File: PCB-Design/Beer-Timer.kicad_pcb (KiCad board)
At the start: 2 copper layers, 47.5 x 19 mm, 19 parts, among them J1 Power, J2 Programmer Pins, J3 TM1637 4 Digit Display, J4 SOIC-ATtiny85-20U, J5 SOIC-2, J6 Switches, SW1 SW_SPDT, U1 MCP1700x-330xxTT, U2 ATtiny85-20S

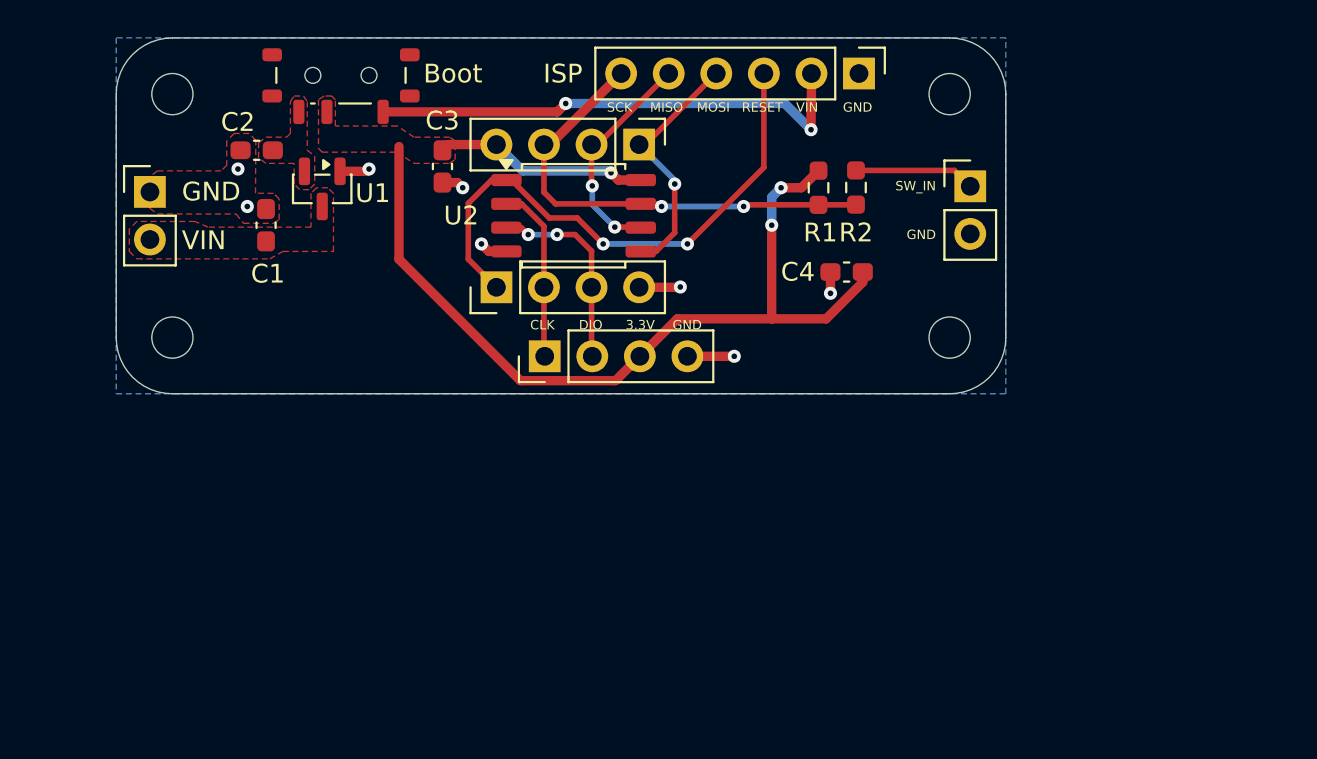
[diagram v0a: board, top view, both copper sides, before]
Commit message: Final PCB changes
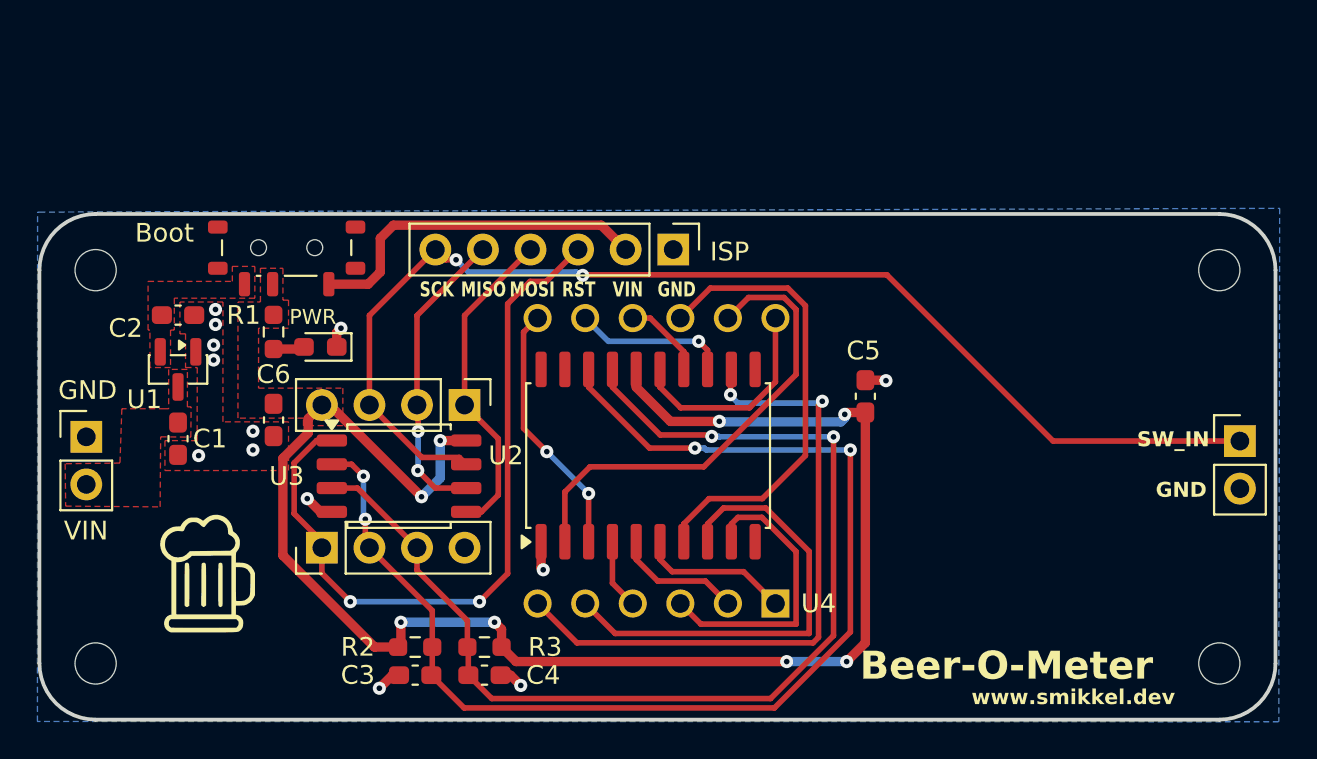
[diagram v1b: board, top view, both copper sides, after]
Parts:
- removed the J3 at (130.9, 86.0)
- added C3: 100p, Capacitor_SMD:C_0603_1608Metric_Pad1.08x0.95mm_HandSolder, F.Cu at (124.0, 103.0)
- added C5: 10uF, Capacitor_SMD:C_0603_1608Metric_Pad1.08x0.95mm_HandSolder, F.Cu at (148.0, 88.1)
- added G***: LOGO, LOGO, F.Cu at (112.8, 97.6)
- added PWR: PWR_LED, LED_SMD:LED_0603_1608Metric_Pad1.05x0.95mm_HandSolder, F.Cu at (118.9, 85.5)
- added R3: 10k, Resistor_SMD:R_0603_1608Metric_Pad0.98x0.95mm_HandSolder, F.Cu at (127.7, 101.5)
- added U2: TM1637, Package_SO:SOP-20_7.5x12.8mm_P1.27mm, F.Cu at (136.4, 91.3)
- added U4: CA56-12EWA, Display_7Segment:CA56-12EWA, B.Cu at (143.2, 99.2)
- C4: value 10uF -> 100p
- R1: value 10k -> 1k
- R2: value 330 -> 10k
- moved H1 63.6 mm to (166.9, 102.4)
- moved H3 46.6 mm to (106.9, 81.4)
- moved R2 34.0 mm to (124.0, 101.5), turned to 0 degrees
- moved R1 30.1 mm to (116.4, 84.7)
- moved C4 28.9 mm to (127.7, 103.0), turned to 0 degrees
- moved J3 19.8 mm to (168.0, 90.5)
- moved H2 17.9 mm to (106.9, 102.4)
- moved J4 16.7 mm to (119.0, 96.2)
- moved J5 16.7 mm to (126.6, 88.6)
- moved U3 16.7 mm to (123.1, 92.4)
- moved C6 16.3 mm to (116.4, 89.4)
- moved H4 14.8 mm to (166.9, 81.4)
- moved J2 13.7 mm to (137.7, 80.3)
- moved J1 13.5 mm to (106.4, 90.3)
- moved U1 12.3 mm to (111.3, 86.7)
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- renumbered C3 to C6, H3 to H2, H2 to H3, J6 to J3, U2 to U3
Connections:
- C4 pad 1: /VCC -> /DIO
- J3 pad 1: Net-(J6-Pin_1) -> /SCK
- R1 pad 2: /SCK -> Net-(D1-A)
- R2 pad 1: /SCK -> /VCC
- R2 pad 2: Net-(J6-Pin_1) -> /CLK
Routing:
- net /CLK: track 9.46 -> 64.9 mm, vias 0 -> 4
- net /DIO: track 10.7 -> 59.7 mm
- net /SCK: track 25.3 -> 63.5 mm
- net /GRID4: track 0.00 -> 35.5 mm, vias 0 -> 2
- net /VCC: track 57.3 -> 83.9 mm, vias 3 -> 8
- net /a: track 0.00 -> 25.4 mm
- net /g: track 0.00 -> 24.7 mm
- net /f: track 0.00 -> 24.7 mm
- net /DPX: track 0.00 -> 15.8 mm
- net /b: track 0.00 -> 13.7 mm, vias 0 -> 2
- net /GRID1: track 0.00 -> 11.6 mm
- net /Reset: track 29.5 -> 39.5 mm
- net /GRID3: track 0.00 -> 8.27 mm, vias 0 -> 1
- net /e: track 0.00 -> 8.09 mm
- net /ISP_VCC: track 26.6 -> 18.7 mm, vias 2 -> 0
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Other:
- board size 47.5 x 19 mm -> 66 x 27 mm
- board text added: "Beer-O-Meter"
- board text added: "RST"
- board text added: "www.smikkel.dev"
- board text removed: "3.3V"
- board text removed: "CLK"
- board text removed: "DIO"
- board text removed: "RESET"
